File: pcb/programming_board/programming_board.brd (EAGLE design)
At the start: 100 x 80 mm, 32 parts

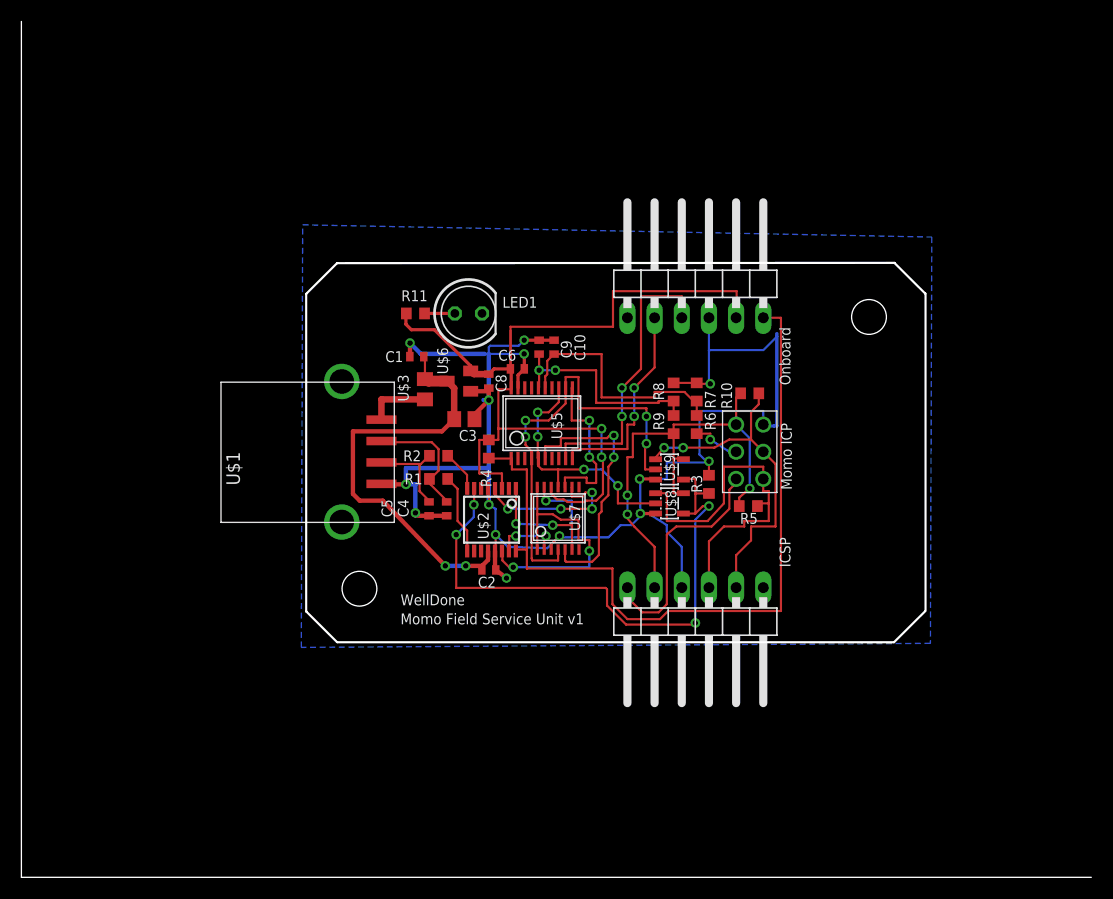
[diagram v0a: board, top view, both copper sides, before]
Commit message: Final version 1.0 of the programming board
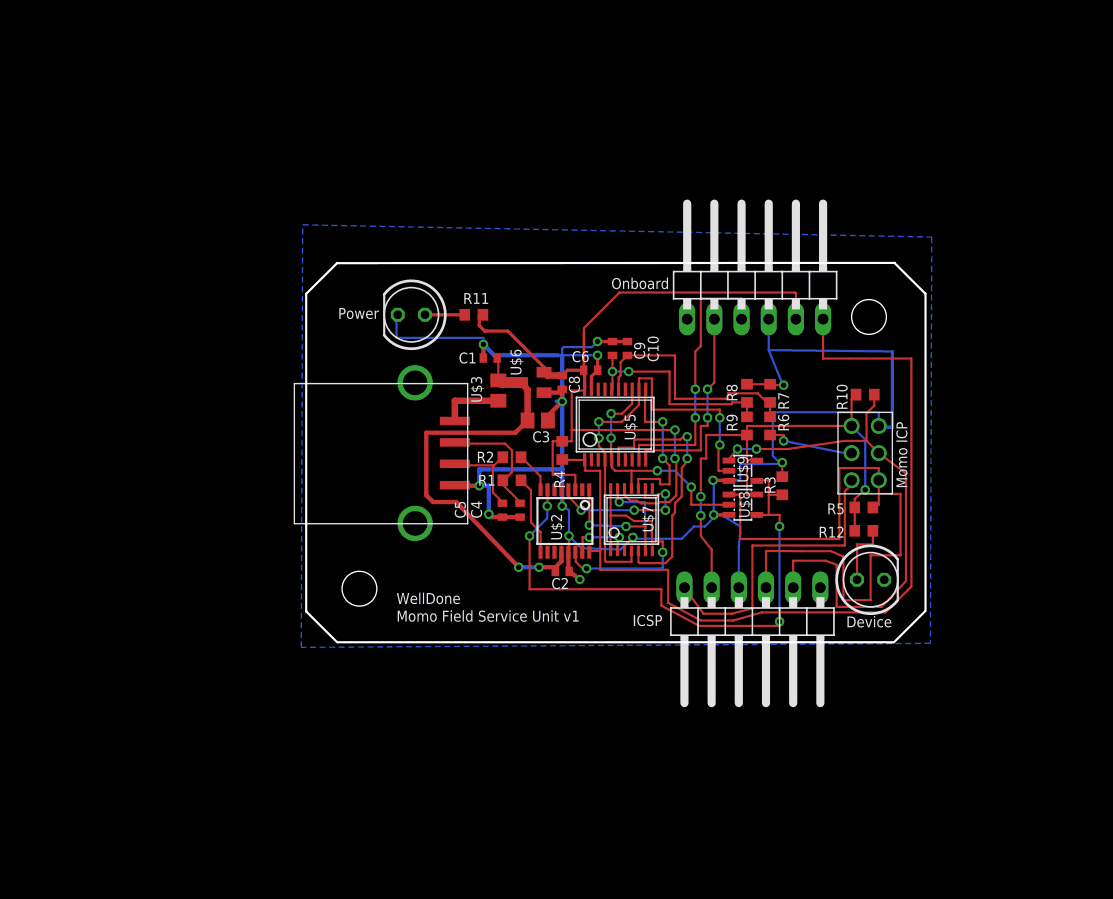
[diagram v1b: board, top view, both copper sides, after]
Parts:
- added LED2: (no value), led:LED5MM
- added R12: 66R, rcl:R0603
- R5: value 19K -> 10K
- moved R10 10.8 mm to (78.9, 45.1)
- moved R5 10.8 mm to (78.7, 34.6)
- moved U$4 10.8 mm to (80.1, 39.6)
- moved C4 6.86 mm to (46.6, 34.3)
- moved C6 6.86 mm to (53.2, 47.4)
- moved R1 6.86 mm to (45.8, 37.1)
- moved R2 6.86 mm to (45.8, 39.3)
- moved R3 6.86 mm to (71.1, 36.6)
- moved R6 6.86 mm to (70.0, 42.2)
- moved R7 6.86 mm to (70.0, 45.2)
- moved U$6 6.86 mm to (47.8, 46.3)
- moved U$7 6.86 mm to (57.0, 33.4)
- moved C10 6.86 mm to (56.6, 49.4)
- moved U$5 6.86 mm to (55.5, 42.3)
- moved C1 6.86 mm to (43.8, 48.5)
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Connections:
- new net N$13: LED2.A, R12.1
- net +3V3: now also R12.2
- net GND: now also LED2.K
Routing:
- net PGD: track 34.6 -> 61.0 mm
- net PGC: track 32.0 -> 51.1 mm
- net GND: track 160.0 -> 177.7 mm
- net N$21: track 72.1 -> 82.0 mm
- net N$6: track 21.9 -> 28.5 mm
- net N$13: track 0.00 -> 6.06 mm
- net +3V3: track 45.6 -> 51.0 mm
- net V+: track 4.57 -> 8.28 mm
- net VCCIO: track 82.3 -> 79.2 mm
- net N$7: track 54.6 -> 53.7 mm
- net N$12: track 2.83 -> 3.72 mm
- net N$9: track 27.0 -> 26.3 mm
- net N$8: track 19.7 -> 19.2 mm
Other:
- board size 100 x 80 mm -> 57.9 x 35.5 mm
- board text added: "Device"
- board text added: "Power"
